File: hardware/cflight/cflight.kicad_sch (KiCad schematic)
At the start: 37 parts, among them J1 7.2v, J2 I2C, J3 3.3v, J4 CH_{1}, J5 GPS connector, J6 GPRS connector, J7 CH_{2}, Q1 BC557, Q2 TIP122, Q3 BC557, Q4 TIP122, U1 ESP32-DEVKIT-V1

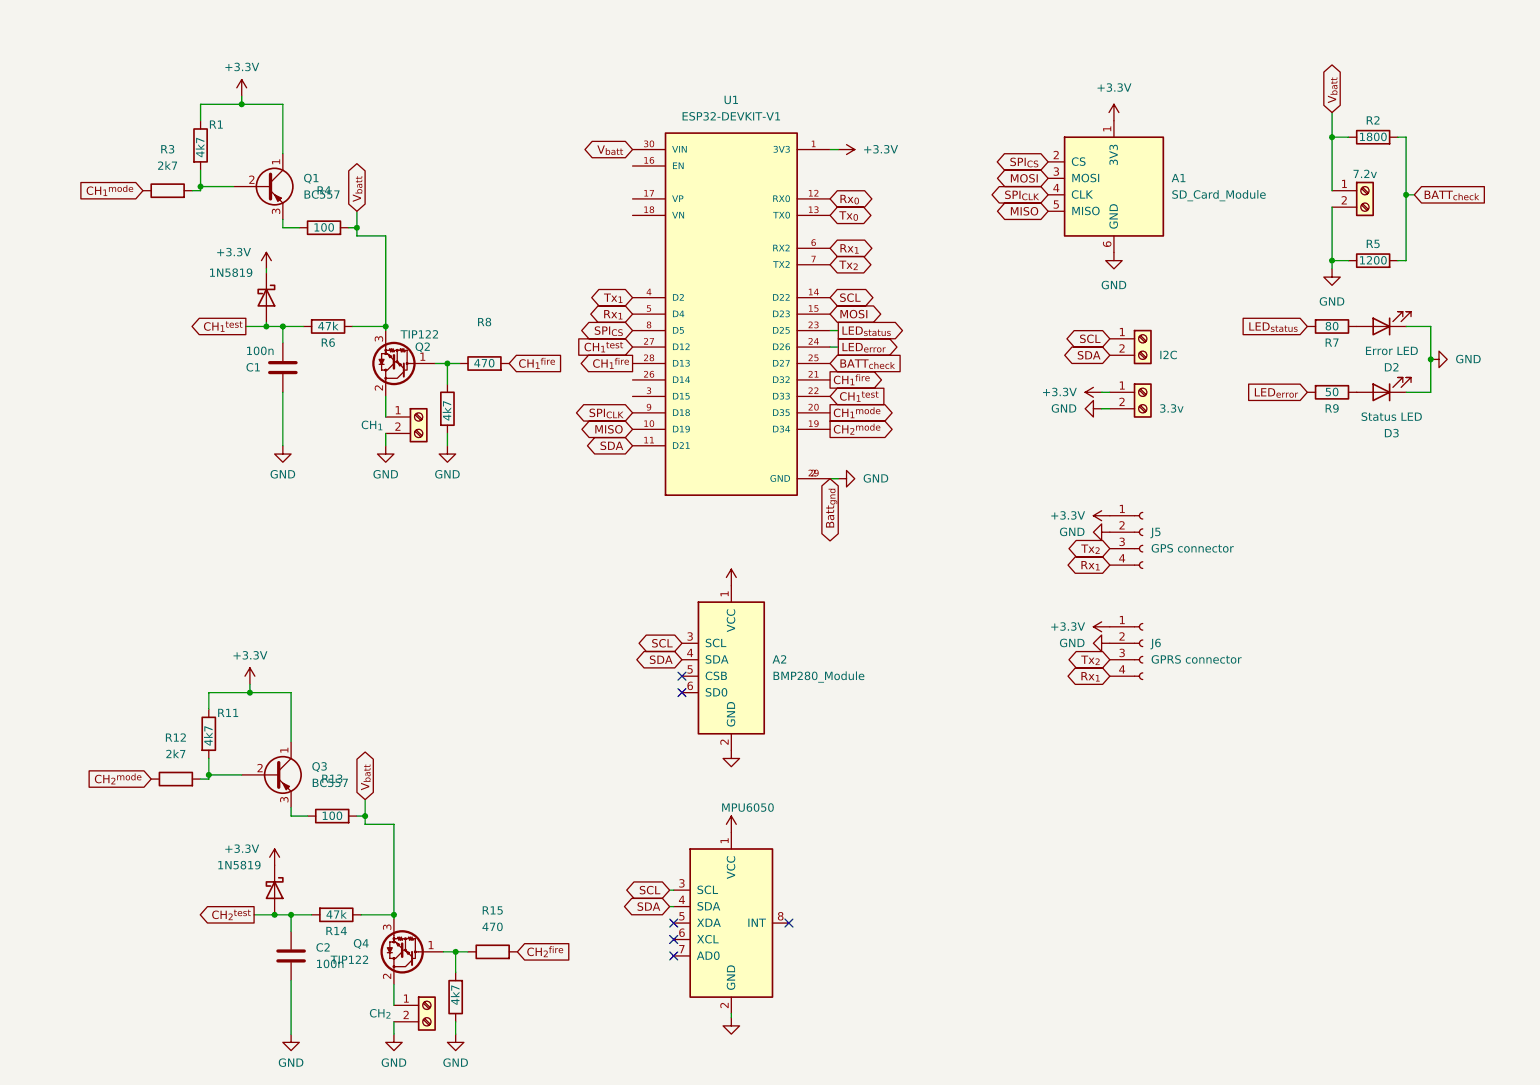
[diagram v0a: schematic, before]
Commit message: college prog
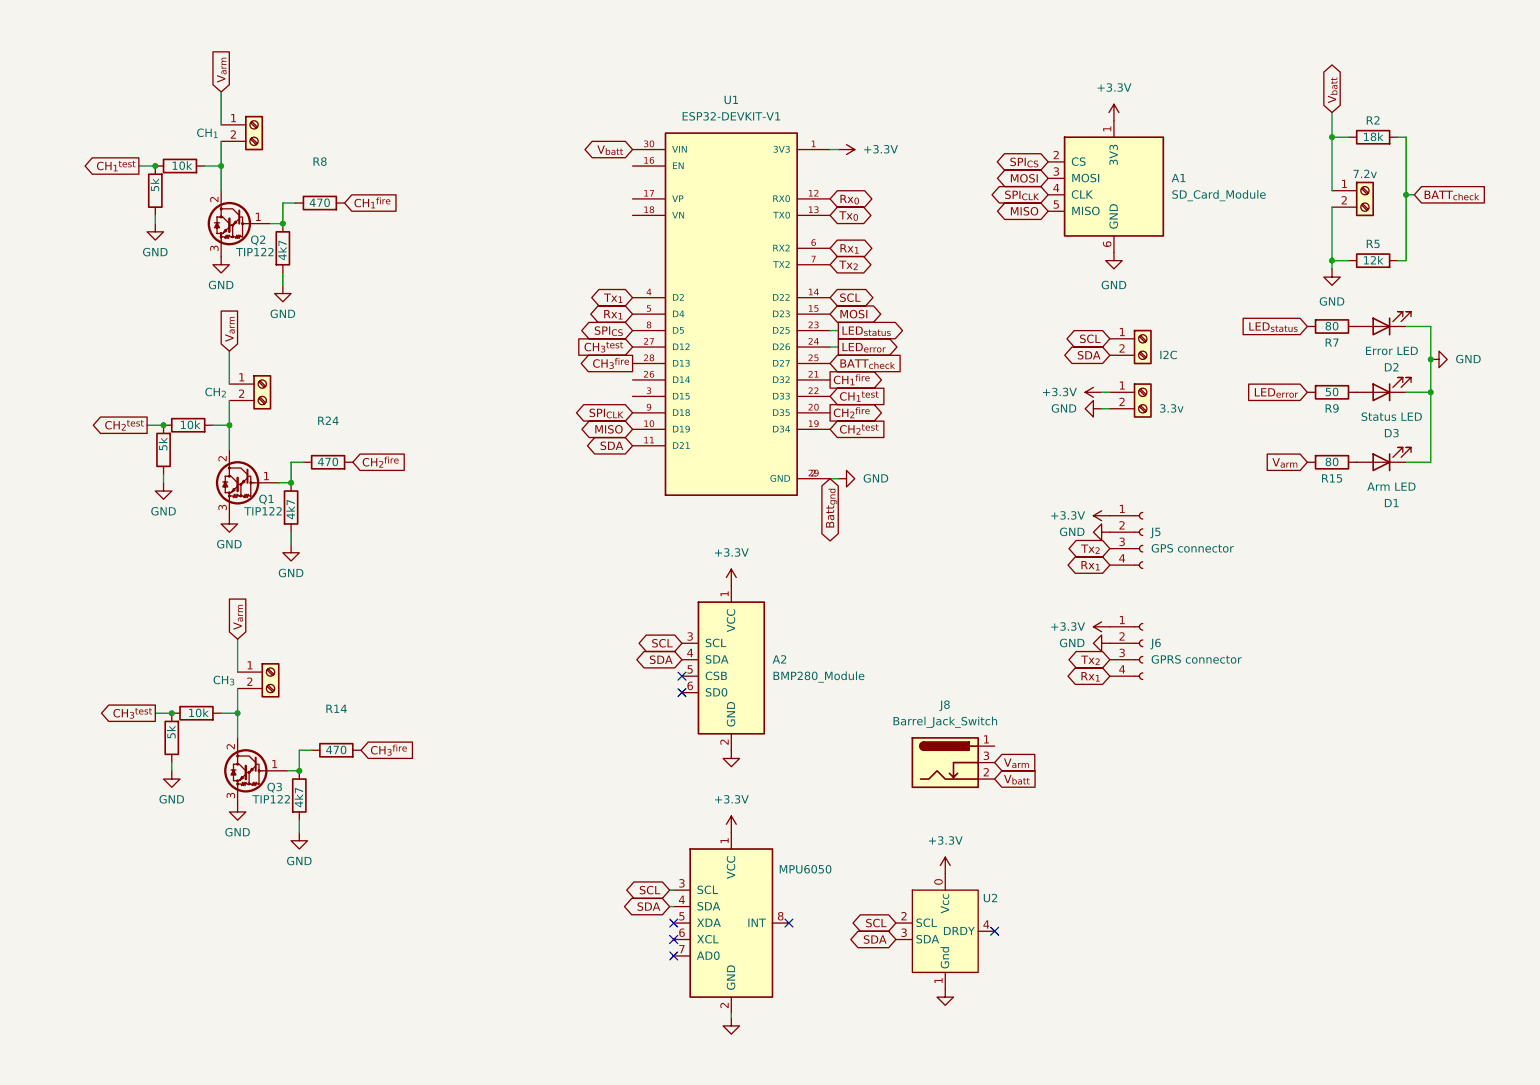
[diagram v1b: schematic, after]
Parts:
- removed C1, C2: 100n, Capacitor_THT:C_Disc_D5.0mm_W2.5mm_P2.50mm, symbol Device:C
- removed D1, D4: 1N5819, Diode_THT:D_DO-41_SOD81_P10.16mm_Horizontal, symbol Diode:1N5819
- removed Q1, Q3: BC557, Package_TO_SOT_THT:TO-92_Inline, symbol Transistor:BC557
- removed Q4: TIP122, Package_TO_SOT_THT:TO-220-3_Vertical, symbol Transistor_BJT:TIP122
- removed R16: 4k7, Resistor_THT:R_Axial_DIN0207_L6.3mm_D2.5mm_P10.16mm_Horizontal, symbol Device:R
- added D1: Arm LED, LED_THT:LED_D3.0mm, symbol Device:LED
- added J10: CH_{2}, TerminalBlock_Phoenix:TerminalBlock_Phoenix_MPT-0,5-2-2.54_1x02_P2.54mm_Horizontal, symbol Connector:Screw_Terminal_01x02
- added J8: Barrel_Jack_Switch, Connector_BarrelJack:BarrelJack_CUI_PJ-063AH_Horizontal, symbol Connector:Barrel_Jack_Switch
- added Q1, Q3: TIP122, Package_TO_SOT_THT:TO-220-3_Vertical, symbol Transistor_BJT:TIP122
- added R23: 4k7, Resistor_THT:R_Axial_DIN0207_L6.3mm_D2.5mm_P10.16mm_Horizontal, symbol Device:R
- added R24: 470, Resistor_THT:R_Axial_DIN0207_L6.3mm_D2.5mm_P10.16mm_Horizontal, symbol Device:R
- added U2: ~, Modules:GY-271, symbol breakouts:GY-271
- J7: value CH_{2} -> CH_{3}
- R1: value 4k7 -> 10k
- R11: value 4k7 -> 5k
- R12: value 2k7 -> 10k
- R13: value 100 -> 4k7
- R14: value 47k -> 470
- R15: value 470 -> 80
- R2: value 1800 -> 18k
- R3: value 2k7 -> 5k
- R4: value 100 -> 5k
- R5: value 1200 -> 12k
- R6: value 47k -> 10k
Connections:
- net +3.3V: now also U2.0 (Vcc); no longer R1.1, R11.1
- net CH_{1}^{fire}: no longer U1.28 (D13)
- net CH_{1}^{test}: now also R1.1, R3.2; no longer R6.2, U1.27 (D12)
- net CH_{2}^{fire}: now also U1.20 (D35), R24.2; no longer R15.2
- net CH_{2}^{test}: now also R4.2, R6.1, U1.19 (D34); no longer R14.2
- net GND: now also Q2.3 (E), R11.1, R13.2, R3.1, R4.1, D1.1 (K), Q1.3 (E), Q3.3 (E), R23.2, U2.1 (Gnd); no longer J4.2 (Pin_2), J7.2 (Pin_2)
- net SCL: now also U2.2 (SCL)
- net SDA: now also U2.3 (SDA)
- net V_{batt}: now also J8.2; no longer Q2.3 (E), R13.2, R14.1, R4.2, R6.1
- net at R1.2: now also J4.2 (Pin_2), Q2.2 (C); no longer R3.2
- net at R15.1: now also D1.2 (A)
- net V_{arm}: now reaches J7.1 (Pin_1)
- net V_{arm}: now also J4.1 (Pin_1), R15.2, J10.1 (Pin_1), J8.3
- net at R12.2: now also J7.2 (Pin_2), Q3.2 (C); no longer R11.2
- net at R13.1: now also R14.1, Q3.1 (B)
- removed net CH_{1}^{mode}: R3.1, U1.20 (D35)
- net CH_{2}^{mode} renamed CH_{3}^{test}
- net CH_{3}^{test}: now also R11.2, U1.27 (D12); no longer U1.19 (D34)
- new net: Q1.1 (B), R23.1, R24.1
- new net: J10.2 (Pin_2), Q1.2 (C), R6.2
- new net CH_{3}^{fire}: R14.2, U1.28 (D13)
- no-connect marks 6 -> 7
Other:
- moved on the sheet: Q2, R8

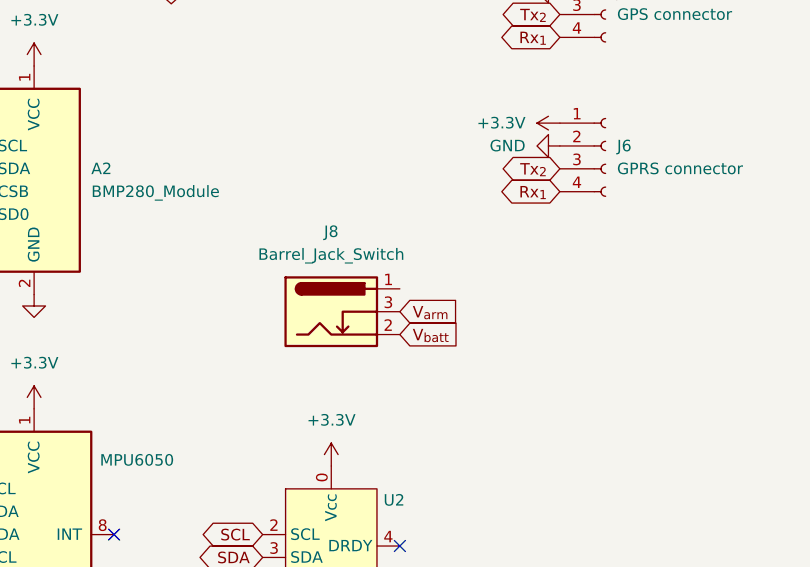
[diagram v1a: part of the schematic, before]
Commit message: Continue hardware
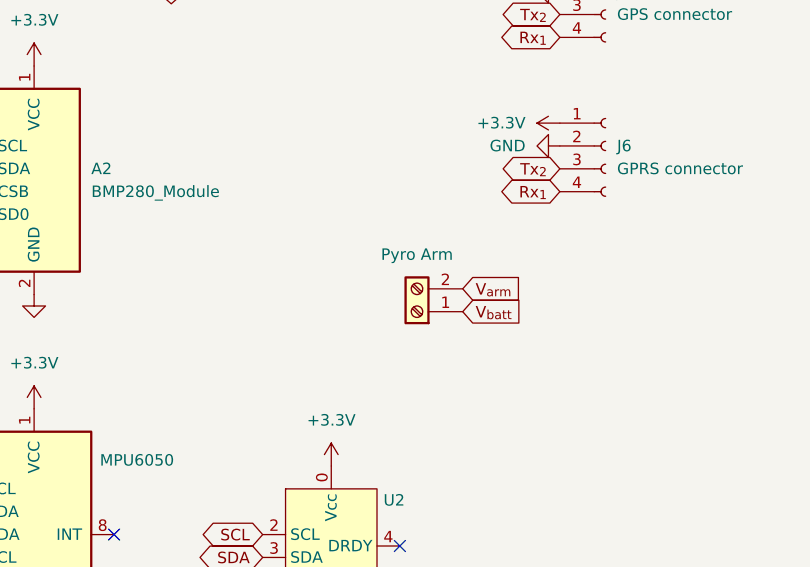
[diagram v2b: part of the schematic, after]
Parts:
- removed J8: Barrel_Jack_Switch, Connector_BarrelJack:BarrelJack_CUI_PJ-063AH_Horizontal, symbol Connector:Barrel_Jack_Switch
- added J?: Pyro Arm, TerminalBlock_Phoenix:TerminalBlock_Phoenix_MPT-0,5-2-2.54_1x02_P2.54mm_Horizontal, symbol Connector:Screw_Terminal_01x02
- D1, D2, D3: footprint LED_THT:LED_D3.0mm -> LED_SMD:LED_0805_2012Metric_Pad1.15x1.40mm_HandSolder
- R1, R10, R11, R12, R13, R14, R15, R2, R23, R24, R3, R4, R5, R6, R7, R8, R9: footprint Resistor_THT:R_Axial_DIN0207_L6.3mm_D2.5mm_P10.16mm_Horizontal -> Resistor_SMD:R_1206_3216Metric_Pad1.30x1.75mm_HandSolder
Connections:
- net V_{arm}: now also J?.2 (Pin_2)
- net V_{batt}: now also J?.1 (Pin_1)
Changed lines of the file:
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@@
     )
   )
-  (global_label "V_{arm}" (shape input) (at 154.94 124.46 0) (fields_autoplaced)
+  (global_label "V_{arm}" (shape input) (at 161.925 121.92 0) (fields_autoplaced)
     (effects (font (size 1.27 1.27)) (justify left))
-    (property "Intersheetrefs" "${INTERSHEET_REFS}" (at 161.8881 124.46 0)
+    (property "Intersheetrefs" "${INTERSHEET_REFS}" (at 168.8731 121.92 0)
       (effects (font (size 1.27 1.27)) (justify left) hide)
     )
@@
     )
   )
-  (global_label "V_{batt}" (shape input) (at 154.94 127 0) (fields_autoplaced)
+  (global_label "V_{batt}" (shape input) (at 161.925 124.46 0) (fields_autoplaced)
     (effects (font (size 1.27 1.27)) (justify left))
-    (property "Intersheetrefs" "${INTERSHEET_REFS}" (at 161.9848 127 0)
+    (property "Intersheetrefs" "${INTERSHEET_REFS}" (at 168.9698 124.46 0)
       (effects (font (size 1.27 1.27)) (justify left) hide)
     )
@@
     )
   )
+  (symbol (lib_id "Connector:Screw_Terminal_01x02") (at 156.845 124.46 180) (unit 1)
+    (in_bom yes) (on_board yes) (dnp no) (fields_autoplaced)
+    (property "Reference" "J?" (at 154.305 124.46 0)
+      (effects (font (size 1.27 1.27)) (justify left) hide)
+    )
+    (property "Value" "Pyro Arm" (at 156.845 118.11 0)
+      (effects (font (size 1.27 1.27)))
+    )
+    (property "Footprint" "TerminalBlock_Phoenix:TerminalBlock_Phoenix_MPT-0,5-2-2.54_1x02_P2.54mm_Horizontal" (at 156.845 124.46 0)
+      (effects (font (size 1.27 1.27)) hide)
+    )
+    (property "Datasheet" "~" (at 156.845 124.46 0)
+      (effects (font (size 1.27 1.27)) hide)
+    )
+    (pin "1")
+    (pin "2")
+    (instances
+      (project "cflight"
+        (path "/96bd4740-d2e5-41ac-9691-b4a6fdf99825"
+          (reference "J?") (unit 1)
+        )
+      )
+    )
+  )
   (symbol (lib_id "Device:R") (at 213.36 46.99 90) (unit 1)
     (in_bom yes) (on_board yes) (dnp no)
@@
       (effects (font (size 1.27 1.27)))
     )
-    (property "Footprint" "Resistor_THT:R_Axial_DIN0207_L6.3mm_D2.5mm_P10.16mm_Horizontal" (at 213.36 48.768 90)
+    (property "Footprint" "Resistor_SMD:R_1206_3216Metric_Pad1.30x1.75mm_HandSolder" (at 213.36 48.768 90)
       (effects (font (size 1.27 1.27)) hide)
     )
@@
       (effects (font (size 1.27 1.27)) (justify left))
     )
-    (property "Footprint" "Resistor_THT:R_Axial_DIN0207_L6.3mm_D2.5mm_P10.16mm_Horizontal" (at 29.21 34.163 90)
+    (property "Footprint" "Resistor_SMD:R_1206_3216Metric_Pad1.30x1.75mm_HandSolder" (at 29.21 34.163 90)
       (effects (font (size 1.27 1.27)) hide)
     )
@@
       (effects (font (size 1.27 1.27)) (justify left))
     )
-    (property "Footprint" "Resistor_THT:R_Axial_DIN0207_L6.3mm_D2.5mm_P10.16mm_Horizontal" (at 45.847 129.54 90)
+    (property "Footprint" "Resistor_SMD:R_1206_3216Metric_Pad1.30x1.75mm_HandSolder" (at 45.847 129.54 90)
       (effects (font (size 1.27 1.27)) hide)
     )
@@
       (effects (font (size 1.27 1.27)))
     )
-    (property "Footprint" "Resistor_THT:R_Axial_DIN0207_L6.3mm_D2.5mm_P10.16mm_Horizontal" (at 207.01 55.372 90)
+    (property "Footprint" "Resistor_SMD:R_1206_3216Metric_Pad1.30x1.75mm_HandSolder" (at 207.01 55.372 90)
       (effects (font (size 1.27 1.27)) hide)
     )
@@
     )
   )
-  (symbol (lib_id "Connector:Barrel_Jack_Switch") (at 147.32 124.46 0) (unit 1)
-    (in_bom yes) (on_board yes) (dnp no) (fields_autoplaced)
-    (property "Reference" "J8" (at 147.32 115.57 0)
-      (effects (font (size 1.27 1.27)))
-    )
-    (property "Value" "Barrel_Jack_Switch" (at 147.32 118.11 0)
-      (effects (font (size 1.27 1.27)))
-    )
-    (property "Footprint" "Connector_BarrelJack:BarrelJack_CUI_PJ-063AH_Horizontal" (at 148.59 125.476 0)
-      (effects (font (size 1.27 1.27)) hide)
-    )
-    (property "Datasheet" "~" (at 148.59 125.476 0)
-      (effects (font (size 1.27 1.27)) hide)
-    )
-    (pin "1")
-    (pin "2")
-    (pin "3")
-    (instances
-      (project "cflight"
-        (path "/96bd4740-d2e5-41ac-9691-b4a6fdf99825"
-          (reference "J8") (unit 1)
-        )
-      )
-    )
-  )
   (symbol (lib_id "Device:LED") (at 214.63 57.15 180) (unit 1)
     (in_bom yes) (on_board yes) (dnp no) (fields_autoplaced)
@@
       (effects (font (size 1.27 1.27)))
     )
-    (property "Footprint" "LED_THT:LED_D3.0mm" (at 214.63 57.15 0)
+    (property "Footprint" "LED_SMD:LED_0805_2012Metric_Pad1.15x1.40mm_HandSolder" (at 214.63 57.15 0)
       (effects (font (size 1.27 1.27)) hide)
     )
@@
       (effects (font (size 1.27 1.27)))
     )
-    (property "Footprint" "Resistor_THT:R_Axial_DIN0207_L6.3mm_D2.5mm_P10.16mm_Horizontal" (at 52.07 79.883 90)
+    (property "Footprint" "Resistor_SMD:R_1206_3216Metric_Pad1.30x1.75mm_HandSolder" (at 52.07 79.883 90)
       (effects (font (size 1.27 1.27)) hide)
     )
@@
       (effects (font (size 1.27 1.27)) (justify left))
     )
-    (property "Footprint" "Resistor_THT:R_Axial_DIN0207_L6.3mm_D2.5mm_P10.16mm_Horizontal" (at 43.307 45.085 90)
+    (property "Footprint" "Resistor_SMD:R_1206_3216Metric_Pad1.30x1.75mm_HandSolder" (at 43.307 45.085 90)
       (effects (font (size 1.27 1.27)) hide)
     )
@@
       (effects (font (size 1.27 1.27)) (justify left))
     )
-    (property "Footprint" "Resistor_THT:R_Axial_DIN0207_L6.3mm_D2.5mm_P10.16mm_Horizontal" (at 27.178 36.195 90)
+    (property "Footprint" "Resistor_SMD:R_1206_3216Metric_Pad1.30x1.75mm_HandSolder" (at 27.178 36.195 90)
       (effects (font (size 1.27 1.27)) hide)
     )
@@
       (effects (font (size 1.27 1.27)))
     )
-    (property "Footprint" "Resistor_THT:R_Axial_DIN0207_L6.3mm_D2.5mm_P10.16mm_Horizontal" (at 207.01 76.327 90)
+    (property "Footprint" "Resistor_SMD:R_1206_3216Metric_Pad1.30x1.75mm_HandSolder" (at 207.01 76.327 90)
       (effects (font (size 1.27 1.27)) hide)
     )
@@
       (effects (font (size 1.27 1.27)) (justify left))
     )
-    (property "Footprint" "Resistor_THT:R_Axial_DIN0207_L6.3mm_D2.5mm_P10.16mm_Horizontal" (at 30.48 74.168 90)
+    (property "Footprint" "Resistor_SMD:R_1206_3216Metric_Pad1.30x1.75mm_HandSolder" (at 30.48 74.168 90)
       (effects (font (size 1.27 1.27)) hide)
     )
@@
       (effects (font (size 1.27 1.27)))
     )
-    (property "Footprint" "Resistor_THT:R_Axial_DIN0207_L6.3mm_D2.5mm_P10.16mm_Horizontal" (at 207.01 65.532 90)
+    (property "Footprint" "Resistor_SMD:R_1206_3216Metric_Pad1.30x1.75mm_HandSolder" (at 207.01 65.532 90)
       (effects (font (size 1.27 1.27)) hide)
     )
@@
       (effects (font (size 1.27 1.27)) (justify left))
     )
-    (property "Footprint" "Resistor_THT:R_Axial_DIN0207_L6.3mm_D2.5mm_P10.16mm_Horizontal" (at 29.718 120.65 90)
+    (property "Footprint" "Resistor_SMD:R_1206_3216Metric_Pad1.30x1.75mm_HandSolder" (at 29.718 120.65 90)
       (effects (font (size 1.27 1.27)) hide)
     )
@@
       (effects (font (size 1.27 1.27)) (justify left))
     )
-    (property "Footprint" "Resistor_THT:R_Axial_DIN0207_L6.3mm_D2.5mm_P10.16mm_Horizontal" (at 44.577 85.09 90)
+    (property "Footprint" "Resistor_SMD:R_1206_3216Metric_Pad1.30x1.75mm_HandSolder" (at 44.577 85.09 90)
       (effects (font (size 1.27 1.27)) hide)
     )
@@
       (effects (font (size 1.27 1.27)) (justify left))
     )
-    (property "Footprint" "Resistor_THT:R_Axial_DIN0207_L6.3mm_D2.5mm_P10.16mm_Horizontal" (at 28.448 76.2 90)
+    (property "Footprint" "Resistor_SMD:R_1206_3216Metric_Pad1.30x1.75mm_HandSolder" (at 28.448 76.2 90)
       (effects (font (size 1.27 1.27)) hide)
     )
@@
       (effects (font (size 1.27 1.27)) (justify left))
     )
-    (property "Footprint" "Resistor_THT:R_Axial_DIN0207_L6.3mm_D2.5mm_P10.16mm_Horizontal" (at 31.75 118.618 90)
+    (property "Footprint" "Resistor_SMD:R_1206_3216Metric_Pad1.30x1.75mm_HandSolder" (at 31.75 118.618 90)
       (effects (font (size 1.27 1.27)) hide)
     )
@@
       (effects (font (size 1.27 1.27)))
     )
-    (property "Footprint" "Resistor_THT:R_Axial_DIN0207_L6.3mm_D2.5mm_P10.16mm_Horizontal" (at 213.36 29.718 90)
+    (property "Footprint" "Resistor_SMD:R_1206_3216Metric_Pad1.30x1.75mm_HandSolder" (at 213.36 29.718 90)
       (effects (font (size 1.27 1.27)) hide)
     )
@@
       (effects (font (size 1.27 1.27)))
     )
-    (property "Footprint" "LED_THT:LED_D3.0mm" (at 214.63 78.105 0)
+    (property "Footprint" "LED_SMD:LED_0805_2012Metric_Pad1.15x1.40mm_HandSolder" (at 214.63 78.105 0)
       (effects (font (size 1.27 1.27)) hide)
     )
@@
       (effects (font (size 1.27 1.27)))
     )
-    (property "Footprint" "LED_THT:LED_D3.0mm" (at 214.63 67.31 0)
+    (property "Footprint" "LED_SMD:LED_0805_2012Metric_Pad1.15x1.40mm_HandSolder" (at 214.63 67.31 0)
       (effects (font (size 1.27 1.27)) hide)
     )
@@
       (effects (font (size 1.27 1.27)))
     )
-    (property "Footprint" "Resistor_THT:R_Axial_DIN0207_L6.3mm_D2.5mm_P10.16mm_Horizontal" (at 53.34 124.333 90)
+    (property "Footprint" "Resistor_SMD:R_1206_3216Metric_Pad1.30x1.75mm_HandSolder" (at 53.34 124.333 90)
       (effects (font (size 1.27 1.27)) hide)
     )
@@
       (effects (font (size 1.27 1.27)))
     )
-    (property "Footprint" "Resistor_THT:R_Axial_DIN0207_L6.3mm_D2.5mm_P10.16mm_Horizontal" (at 50.8 39.878 90)
-      (effects (font (size 1.27 1.27)) hide)
-    )
+    (property "Footprint" "Resistor_SMD:R_1206_3216Metric_Pad1.30x1.75mm_HandSolder" (at 50.8 39.878 90)
+      (effects (font (size 1.27 1.27)) hide)
+    )
